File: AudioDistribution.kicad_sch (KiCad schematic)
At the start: 22 parts, among them K1 JW2, K2 JW2, K3 JW2, K4 JW2, K5 JW2, U3 LM7805

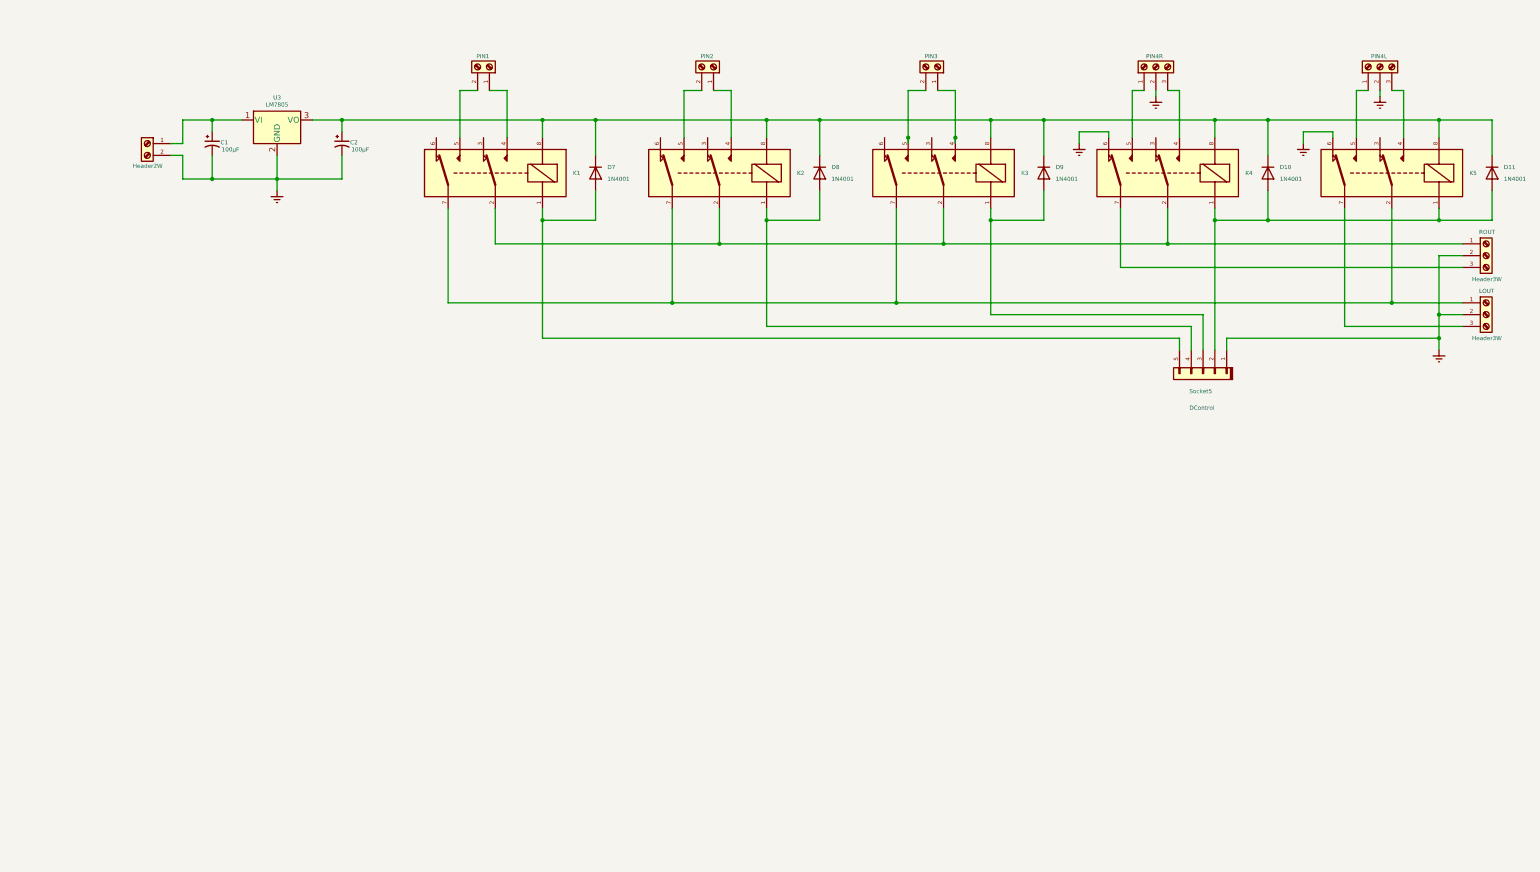
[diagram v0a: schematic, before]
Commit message: Completed Schematics :
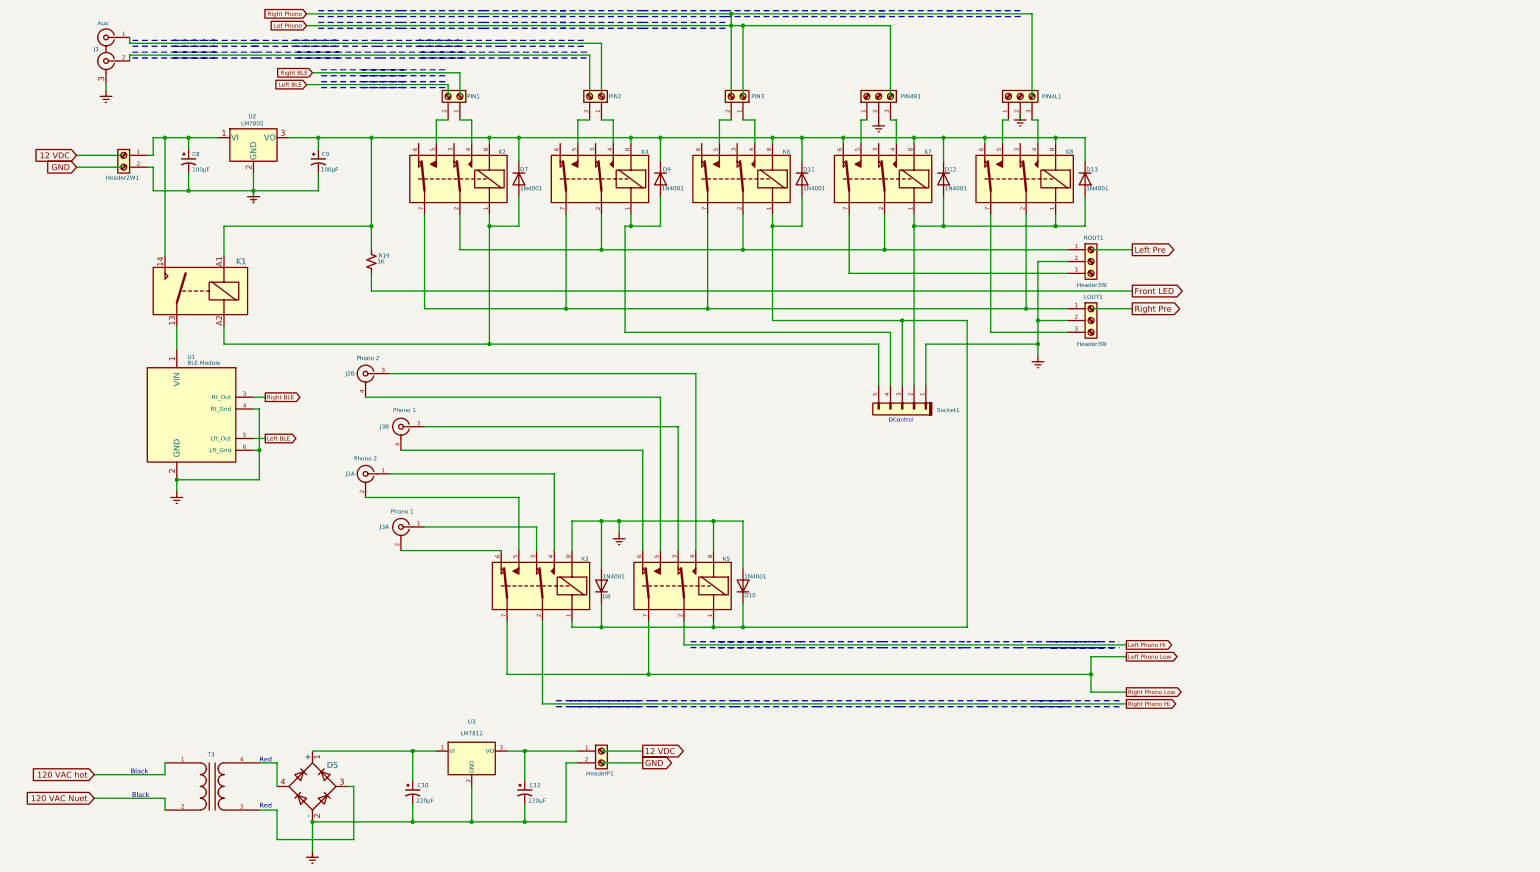
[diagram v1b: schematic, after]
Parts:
- removed D11: 1N4001, Diode_THT:D_DO-41_SOD81_P10.16mm_Horizontal, symbol Diode:1N4001
- removed K2: JW2, Relay_THT:Relay_DPDT_Panasonic_JW2, symbol Relay:JW2
- added C10, C12: 220µF, symbol Device:C_Polarized_Small_US
- added D12, D13, D9: 1N4001, Diode_THT:D_DO-41_SOD81_P10.16mm_Horizontal, symbol Diode:1N4001
- added D5: ABS2, Diode_SMD:Diode_Bridge_Diotec_ABS, symbol Diode_Bridge:ABS2
- added HeaderP1: Screw_Terminal_01x02, symbol Connector:Screw_Terminal_01x02
- added J1: Aux, symbol Connector:Conn_Coaxial_x2
- added J2: Phono 2, symbol Connector:Conn_Coaxial_x2_Isolated
- added J3: Phono 1, symbol Connector:Conn_Coaxial_x2_Isolated
- added K1: Fujitsu_FTR-LYAA005x, Relay_THT:Relay_SPST-NO_Fujitsu_FTR-LYAA005x_FormA_Vertical, symbol Relay:Fujitsu_FTR-LYAA005x
- added K6, K7, K8: JW2, Relay_THT:Relay_DPDT_Panasonic_JW2, symbol Relay:JW2
- added R19: 1K, symbol Resistors:R_Small_US
- added T3: ~, symbol Device:Transformer_1P_1S
- added U1: BLE Module, symbol RF_Bluetooth:SPBTLE-RF
- added U3: LM7812, Package_TO_SOT_THT:TO-220-3_Vertical, symbol Regulator_Linear:LM7812_TO220
- renumbered C1 to C8, C2 to C9, D9 to D11, Header2W to Header2W1, K1 to K2, LOUT to LOUT1, PIN4L to PIN4L1, PIN4R to PIN4R1, ROUT to ROUT1, Socket5 to Socket1, U3 to U2
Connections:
- net GNDREF: now also D10.2 (A), D8.2 (A), K3.8, K5.8, C10.2, C12.2, D5.2 (-), HeaderP1.2 (Pin_2), J1.3 (EXT), U1.2 (GND), U1.4 (Rt_Gnd), U1.6 (Lft_Gnd), U3.2 (GND); no longer K4.6, K5.6
- net at K2.7, LOUT1.1 (Pin_1): now also K4.7, K6.7, K8.2; no longer K3.7, K5.2
- net at K5.3: now also J3.3 (In2)
- net at PIN4L1.3 (Pin_3): now also K8.4; no longer K5.4
- net at PIN4L1.1 (Pin_1): now also K8.5; no longer K5.5
- net at LOUT1.3 (Pin_3): now also K8.7; no longer K5.7
- net at C9.1, D11.1 (K), D7.1 (K)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: now also D12.1 (K), D13.1 (K), D9.1 (K), K1.A1, K6.8, K7.6, K7.8, K8.6, K8.8, R19.1; no longer D10.1 (K), D8.1 (K), K3.8, K5.8
- net at D11.2 (A), K3.1, Socket1.3 (Pin_3): now also D10.1 (K), D8.1 (K), K5.1, K6.1
- net at Socket1.4 (Pin_4): now also K4.1, D9.2 (A); no longer D8.2 (A)
- net at D7.2 (A), K2.1, Socket1.5 (Pin_5): now also K1.A2
- net at C8.1, Header2W1.1 (Pin_1), U2.1 (VI): now also K1.14
- net at K2.2, K4.2, ROUT1.1 (Pin_1): now also K6.2, K7.2; no longer K3.2
- net at PIN2.1 (Pin_1): now also K4.4
- net at PIN2.2 (Pin_2): now also K4.5
- net at K3.3: now also J3.1 (In1)
- net at K3.4: now also J2.1 (In1); no longer PIN3.1 (Pin_1)
- net at K3.5: now also J2.2 (Ext1); no longer PIN3.2 (Pin_2)
- net at K3.6: now also J3.2 (Ext1)
- net at ROUT1.3 (Pin_3): now also K7.7; no longer K4.7
- net at PIN4R1.3 (Pin_3): now also K7.4; no longer K4.4
- net at PIN4R1.1 (Pin_1): now also K7.5; no longer K4.5
- new net: C10.1, D5.1 (+), U3.1 (VI)
- new net: D5.3, T3.3 (SA)
- new net: D5.4, T3.4 (SB)
- new net: D12.2 (A), D13.2 (A), K7.1, K8.1, Socket1.2 (Pin_2)
- new net: J3.4 (Ext2), K5.6
- new net: C12.1, HeaderP1.1 (Pin_1), U3.3 (VO)
- new net: K1.13, U1.1 (VIN)
- new net: K6.4, PIN3.1 (Pin_1)
- new net: K6.5, PIN3.2 (Pin_2)
- new net: J2.3 (In2), K5.4
- new net: J2.4 (Ext2), K5.5
- new net 120 VAC Nuet: T3.2 (AB)
- new net 120 VAC hot: T3.1 (AA)
- new net Front LED: R19.2
- new net Left BLE: U1.5 (Lft_Out)
- new net Left Phono Hi: K5.2
- new net Left Phono Low: K3.7, K5.7
- new net Right BLE: U1.3 (Rt_Out)
- new net Right Phono Hi: K3.2
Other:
- note added: "Black"
- note added: "Red"
- moved on the sheet: C8, C9, D11, Header2W1, LOUT1, PIN1, PIN2, PIN3, PIN4L1, PIN4R1, ROUT1, Socket1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
